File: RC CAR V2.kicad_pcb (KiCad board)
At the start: 2 copper layers, 65 x 65 mm, 62 parts, among them J2 IR1, J3 IR2, J5 US, J6 LW, J7 RW, Q1 S8050, Q2 S8050, SW1 EN, SW2 BOOT, U1 L7805, U2 SRV05-4, U3 AMS1117-3.3, U4 CH340K, U6 L293DD, U7 ESP32-WROOM-32D

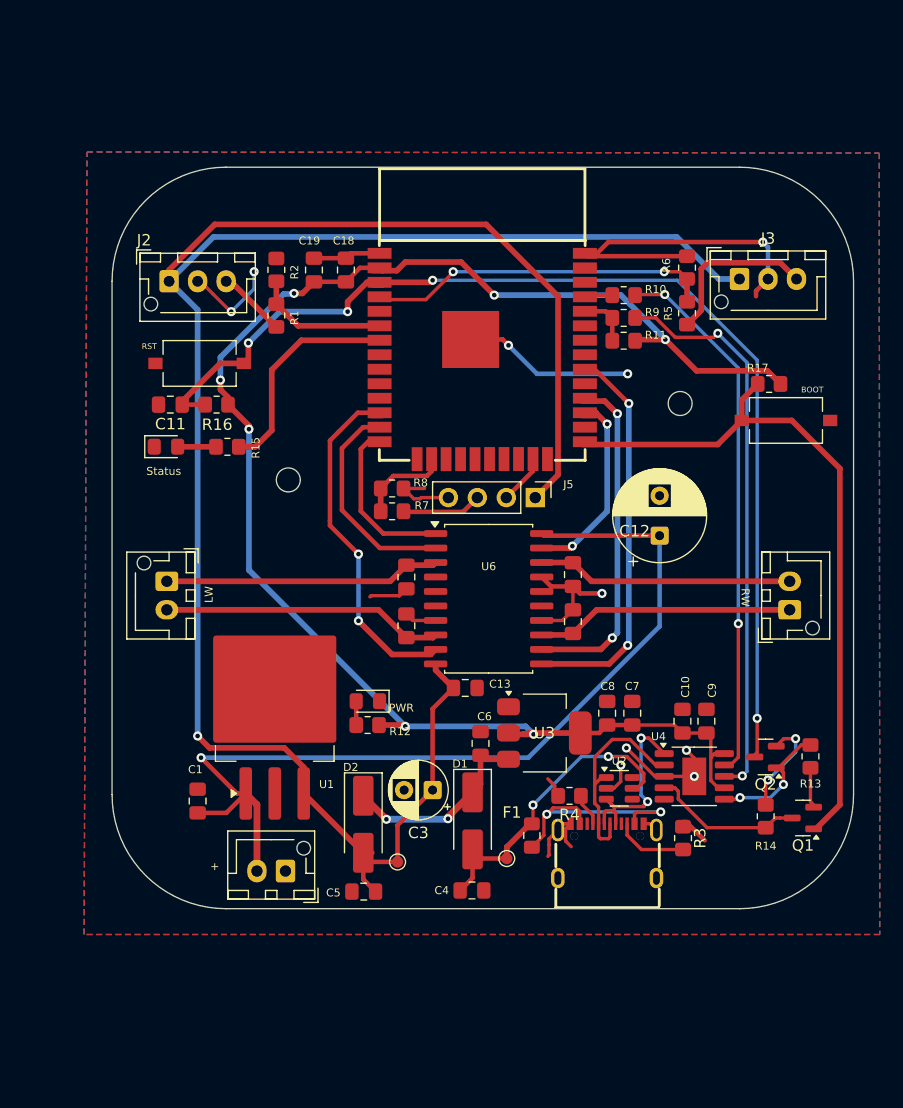
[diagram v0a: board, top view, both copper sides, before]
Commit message: Version of the RC_CAR Circuit Routing Done
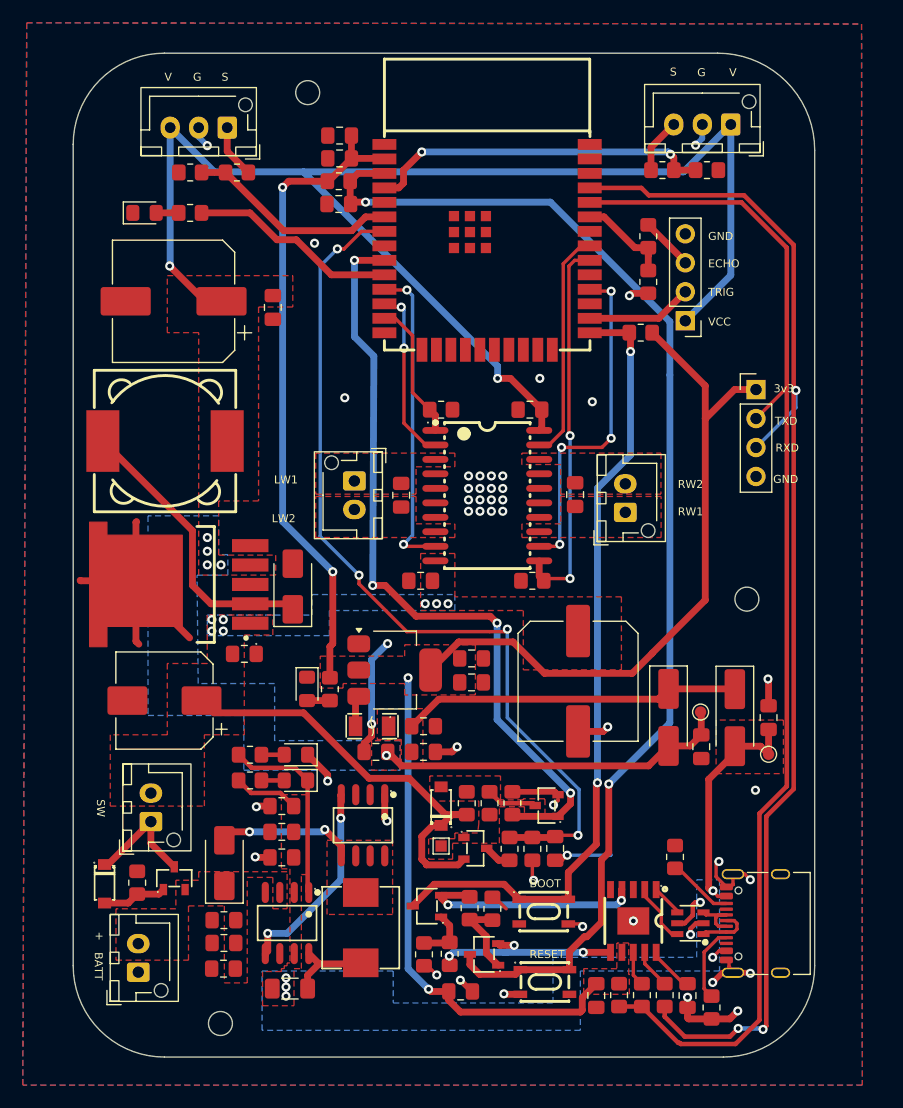
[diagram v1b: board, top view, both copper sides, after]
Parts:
- removed H1: MountingHole, MountingHole:MountingHole_2.1mm
- removed Q2: S8050, Package_TO_SOT_SMD:SOT-23
- removed R3, R4: 5k1, Resistor_SMD:R_0805_2012Metric_Pad1.20x1.40mm_HandSolder
- removed SW1: EN, Button_Switch_SMD:SW_Tactile_SPST_NO_Straight_CK_PTS636Sx25SMTRLFS
- removed SW2: BOOT, Button_Switch_SMD:SW_Tactile_SPST_NO_Straight_CK_PTS636Sx25SMTRLFS
- removed U7: ESP32-WROOM-32D, EasyEDA:WIFIM-SMD_39P-L25.5-W18.0-P1.27-BL
- removed USB1: TYPE-C 16PIN 2MD, EasyEDA:USB-C-SMD_TYPE-C-16PIN-2MD-073
- added C2: 22uF, Capacitor_SMD:C_0805_2012Metric_Pad1.18x1.45mm_HandSolder, F.Cu at (128.8, 120.6)
- added C20: 100nF, Capacitor_SMD:C_0805_2012Metric_Pad1.18x1.45mm_HandSolder, F.Cu at (150.6, 83.6)
- added C21: 22uF, Capacitor_SMD:C_0805_2012Metric_Pad1.18x1.45mm_HandSolder, F.Cu at (133.9, 59.6)
- added C22: 100nF, Capacitor_SMD:C_0805_2012Metric_Pad1.18x1.45mm_HandSolder, F.Cu at (154.5, 91.0)
- added C23: 1uF, Capacitor_SMD:C_0805_2012Metric_Pad1.18x1.45mm_HandSolder, F.Cu at (133.8, 65.6)
- added C24: 100nF, Capacitor_SMD:C_0805_2012Metric_Pad1.18x1.45mm_HandSolder, F.Cu at (139.3, 91.1)
- added C25: 22u, Capacitor_SMD:C_0805_2012Metric_Pad1.18x1.45mm_HandSolder, F.Cu at (171.5, 110.6)
- added C26: 100nF, Capacitor_SMD:C_0805_2012Metric_Pad1.18x1.45mm_HandSolder, F.Cu at (144.5, 134.6)
- added C27: 100nF, Capacitor_SMD:C_0805_2012Metric_Pad1.18x1.45mm_HandSolder, F.Cu at (156.4, 135.0)
- added C28: 22u, Capacitor_SMD:C_0805_2012Metric_Pad1.18x1.45mm_HandSolder, F.Cu at (165.6, 113.1)
- added C32: 100nF, Capacitor_SMD:C_0805_2012Metric_Pad1.18x1.45mm_HandSolder, F.Cu at (164.4, 135.0)
- added D10: SS34, Diode_SMD:D_SMA_Handsoldering, F.Cu at (168.5, 110.6)
- added D11: SS34, Diode_SMD:D_SMA_Handsoldering, F.Cu at (162.7, 110.6)
- added D5: SS34, Diode_SMD:D_SMA, F.Cu at (123.8, 123.3)
- added D6: LED, LED_SMD:LED_0805_2012Metric_Pad1.15x1.40mm_HandSolder, F.Cu at (131.0, 108.1)
- added D7: LED, LED_SMD:LED_0805_2012Metric_Pad1.15x1.40mm_HandSolder, F.Cu at (116.8, 66.3)
- added H2: MountingHole, MountingHole:MountingHole_2.1mm, F.Cu at (169.6, 100.2)
- added H3: MountingHole, MountingHole:MountingHole_2.1mm, F.Cu at (131.1, 55.8)
- added J1: USB_C_Receptacle_USB2.0_16P, Connector_USB:USB_C_Receptacle_Palconn_UTC16-G, F.Cu at (170.3, 128.6)
- added J4: US, Connector_PinHeader_2.54mm:PinHeader_1x04_P2.54mm_Vertical, F.Cu at (164.2, 75.8)
- added L1: CDRH127N-470M, EasyEDA:IND-SMD_L12.3-W12.3, F.Cu at (118.6, 86.3)
- added L2: MHCI06030-4R7M-R8, EasyEDA:IND-SMD_L7.3-W6.6_MHCI06030, F.Cu at (135.8, 129.0)
- added Q3: AO3401A, EasyEDA:SOT-23-3_L2.9-W1.3-P1.90-LS2.4-BR, F.Cu at (145.8, 122.0)
- added Q4: AO3400A, EasyEDA:SOT-23-3_L2.9-W1.3-P1.90-LS2.4-BR, F.Cu at (152.0, 118.3)
- added Q5: S8050H 200-350, EasyEDA:SOT-23-3_L2.9-W1.6-P1.90-LS2.8-BR, F.Cu at (141.6, 127.1)
- added Q6: S8050H 200-350, EasyEDA:SOT-23-3_L2.9-W1.6-P1.90-LS2.8-BR, F.Cu at (146.6, 131.3)
- added Q7: AO3401A, EasyEDA:SOT-23-3_L2.9-W1.3-P1.90-LS2.4-BR, F.Cu at (119.4, 124.7)
- added R18: 1k, Resistor_SMD:R_0805_2012Metric_Pad1.20x1.40mm_HandSolder, F.Cu at (124.9, 62.8)
- added R19: 2k, Resistor_SMD:R_0805_2012Metric_Pad1.20x1.40mm_HandSolder, F.Cu at (120.8, 62.8)
- added R20: 33R, Resistor_SMD:R_0805_2012Metric_Pad1.20x1.40mm_HandSolder, F.Cu at (160.4, 134.9)
- added R21: 33R, Resistor_SMD:R_0805_2012Metric_Pad1.20x1.40mm_HandSolder, F.Cu at (162.4, 134.9)
- added R22: 1k, Resistor_SMD:R_0805_2012Metric_Pad1.20x1.40mm_HandSolder, F.Cu at (161.0, 68.4)
- added R23: 2k, Resistor_SMD:R_0805_2012Metric_Pad1.20x1.40mm_HandSolder, F.Cu at (161.0, 72.4)
- added R24: 100K, Resistor_SMD:R_0805_2012Metric_Pad1.20x1.40mm_HandSolder, F.Cu at (147.3, 127.3)
- added R25: 100K, Resistor_SMD:R_0805_2012Metric_Pad1.20x1.40mm_HandSolder, F.Cu at (141.3, 131.3)
- added R26: 10k, Resistor_SMD:R_0805_2012Metric_Pad1.20x1.40mm_HandSolder, F.Cu at (158.4, 134.9)
- added R27: 10K, Resistor_SMD:R_0805_2012Metric_Pad1.20x1.40mm_HandSolder, F.Cu at (143.5, 131.3)
- added R28: 10K, Resistor_SMD:R_0805_2012Metric_Pad1.20x1.40mm_HandSolder, F.Cu at (145.3, 127.3)
- added R29: 5k1, Resistor_SMD:R_0805_2012Metric_Pad1.20x1.40mm_HandSolder, F.Cu at (163.3, 122.8)
- added R30: 10k, Resistor_SMD:R_0805_2012Metric_Pad1.20x1.40mm_HandSolder, F.Cu at (142.8, 83.6)
- added R31: 10k, Resistor_SMD:R_0805_2012Metric_Pad1.20x1.40mm_HandSolder, F.Cu at (150.8, 98.6)
- added R32: 5k1, Resistor_SMD:R_0805_2012Metric_Pad1.20x1.40mm_HandSolder, F.Cu at (166.5, 136.0)
- added SW3: BOOT, EasyEDA:SW-SMD_4P-L4.2-W3.4-P2.15-LS5.2, F.Cu at (151.8, 127.6)
- added SW4: EN, EasyEDA:SW-SMD_4P-L4.2-W3.4-P2.15-LS5.2, F.Cu at (151.9, 133.8)
- added Switch_Connector1: J3, Connector_JST:JST_XH_B2B-XH-AM_1x02_P2.50mm_Vertical, F.Cu at (117.4, 119.7)
- added TP4: TestPoint, TestPoint:TestPoint_Pad_D1.0mm, F.Cu at (165.5, 110.1)
- added U5: L293DDM/TR, EasyEDA:SOP-20_L12.8-W7.5-P1.27-LS10.4-BL, F.Cu at (146.8, 91.1)
- added ZD1: BZT52C10, EasyEDA:SOD-123_L2.8-W1.8-LS3.7-RD, F.Cu at (142.8, 118.3)
- added ZD2: BZT52C10, EasyEDA:SOD-123_L2.8-W1.8-LS3.7-RD, F.Cu at (113.3, 125.2)
- C1, C10, C16, C9: value 0.1uF -> 22uF
- C11: value 0.1uF -> 22u
- C12: value 470uF -> 10uF; footprint Capacitor_THT:CP_Radial_D8.0mm_P3.50mm -> Capacitor_SMD:C_0805_2012Metric_Pad1.18x1.45mm_HandSolder
- C13, C14, C15, C18: value 0.1uF -> 100nF
- C17: value 0.1uF -> 470uF; footprint Capacitor_SMD:C_0805_2012Metric_Pad1.18x1.45mm_HandSolder -> Capacitor_SMD:C_Elec_10x10.2
- C19: value 22uF -> 100nF
- C3: value CPS -> 100uF; footprint Capacitor_THT:CP_Radial_D5.0mm_P2.50mm -> Capacitor_SMD:CP_Elec_8x10
- C4, C8: value 22u -> 22uF
- C5: value 22u -> 100nF
- C6: value 10u -> 330uF; footprint Capacitor_SMD:C_0805_2012Metric_Pad1.18x1.45mm_HandSolder -> Capacitor_SMD:CP_Elec_10x10.5
- C7: value 0.1u -> 100nF
- D1: value SS34 -> R_LED; footprint Diode_SMD:D_SMA_Handsoldering -> LED_SMD:LED_0805_2012Metric_Pad1.15x1.40mm_HandSolder
- D2: value SS34 -> G_LED; footprint Diode_SMD:D_SMA_Handsoldering -> LED_SMD:LED_0805_2012Metric_Pad1.15x1.40mm_HandSolder
- D3: value LED -> SS34; footprint LED_SMD:LED_0805_2012Metric_Pad1.15x1.40mm_HandSolder -> Diode_SMD:D_SMA
- D4: value LED -> USBLC6-2SC6; footprint LED_SMD:LED_0805_2012Metric_Pad1.15x1.40mm_HandSolder -> EasyEDA:SOT-23-6_L2.9-W1.6-P0.95-LS2.8-BL
- F1: value Polyfuse_Small -> SMD1206P100TF; footprint Fuse:Fuse_0805_2012Metric_Pad1.15x1.40mm_HandSolder -> EasyEDA:F1206
- J5: value US -> LW; footprint Connector_PinHeader_2.54mm:PinHeader_1x04_P2.54mm_Vertical -> Connector_JST:JST_XH_B2B-XH-AM_1x02_P2.50mm_Vertical
- J6: value LW -> RW
- J7: value RW -> Progmmer; footprint Connector_JST:JST_XH_B2B-XH-AM_1x02_P2.50mm_Vertical -> Connector_PinHeader_2.54mm:PinHeader_1x04_P2.54mm_Vertical
- Q1: value S8050 -> AO4468; footprint Package_TO_SOT_SMD:SOT-23 -> EasyEDA:SOP-8_L4.9-W3.9-P1.27-LS6.0-BL
- R1: value 1k -> 4k7
- R10, R9: value 33R -> 10K
- R11: value 10k -> 10K
- R13: value 10K -> 1k
- R14: value 10K -> 10k
- R15: value 1k -> 10k
- R16: value 10k -> 1k
- R17: value 10k -> 2k
- R2: value 2k -> 4k7
- R5: value 1k -> R040; footprint Resistor_SMD:R_0805_2012Metric_Pad1.20x1.40mm_HandSolder -> Resistor_SMD:R_1206_3216Metric_Pad1.30x1.75mm_HandSolder
- R6: value 2k -> 1K
- R7: value 1k -> 430K
- R8: value 2k -> 100K
- TP2: footprint TestPoint:TestPoint_Pad_D1.0mm -> TestPoint:TestPoint_Pad_1.0x1.0mm
- U1: value L7805 -> LM2596SX-5.0/NOPB; footprint Package_TO_SOT_SMD:TO-263-3_TabPin2 -> EasyEDA:TO-263-5_L10.2-W8.9-P1.70-TL
- U2: value SRV05-4 -> CN3303; footprint Package_TO_SOT_SMD:SOT-23-6 -> EasyEDA:SOP-8_L4.9-W3.9-P1.27-LS6.0-BL-1
- U4: value CH340K -> ESP32-WROOM-32E-N8R2; footprint Package_SO:SSOP-10-1EP_3.9x4.9mm_P1mm_EP2.1x3.3mm -> EasyEDA:WIFI-SMD_ESP32-WROOM-32E
- U6: value L293DD -> CH340K; footprint Package_SO:SOIC-20W_7.5x12.8mm_P1.27mm -> EasyEDA:ESOP-10_L4.9-W3.9-P1.00-LS6.2-BL-EP
- moved R6 72.3 mm to (116.2, 125.1)
- moved R13 72.3 mm to (120.8, 66.3), turned to 180 degrees
- moved R5 68.7 mm to (129.5, 134.3), turned to 0 degrees
- moved R14 67.1 mm to (133.8, 63.6), turned to 0 degrees
- moved D4 62.1 mm to (164.6, 128.6), turned to 90 degrees
- moved J2 51.1 mm to (168.2, 58.6), turned to 180 degrees
- moved U4 49.8 mm to (146.8, 69.3), turned to -90 degrees
- moved H4 48.0 mm to (123.5, 137.4)
- moved C7 47.5 mm to (128.0, 74.6)
- moved C6 47.2 mm to (119.3, 74.1), turned to 180 degrees
- moved J3 46.8 mm to (124.0, 58.9), turned to 180 degrees
- moved C9 46.5 mm to (123.8, 130.3), turned to 180 degrees
- moved R10 46.1 mm to (147.0, 118.1), turned to 90 degrees
- moved R9 44.7 mm to (145.0, 118.1), turned to 90 degrees
- moved R16 44.2 mm to (162.2, 62.6), turned to 0 degrees
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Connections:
- BATT1 pad 2: +12V -> /BATT+
- C1 pad 1: +12V -> VBUS
- C10 pad 1: +3.3V -> /BATT+
- C11 pad 1: EN -> +5V
- C12 pad 1: +12V -> V-IN
- C13 pad 1: +5V -> BATT_ADC
- C14 pad 1: RW1 -> V-IN
- C15 pad 1: RW2 -> +3.3V
- C16 pad 1: LW1 -> +3.3V
- C17 pad 1: LW2 -> +12V
- C18 pad 1: +3.3V -> +12V
- C3 pad 1: +5V -> +12V
- C5 pad 1: +5V -> +12V
- C6 pad 1: V-IN -> +5V
- C7 pad 1: +3.3V -> GND
- C7 pad 2: GND -> +5V
- C8 pad 1: +3.3V -> /BATT+
- C9 pad 1: +3.3V -> /BATT+
- D1 pad 1: V-IN -> Net-(D1-K)
- D1 pad 2: VBUS -> Net-(D1-A)
- D2 pad 1: V-IN -> GND
- D2 pad 2: +5V -> Net-(D2-A)
- D3 pad 1: GND -> Net-(D3-K)
- D3 pad 2: Net-(D3-A) -> GND
- D4 pad 1: GND -> D-
- D4 pad 2: Net-(D4-A) -> GND
- F1 pad 1: VBUS -> V-IN
- F1 pad 2: Net-(F1-Pad2) -> Net-(U3-VI)
- J3 pad 1: +5V -> Net-(J3-Pin_1)
- J3 pad 3: Net-(J3-Pin_3) -> +5V
- J5 pad 1: +5V -> LW1
- J5 pad 2: TRIG -> LW2
- J6 pad 1: LW1 -> RW1
- J6 pad 2: LW2 -> RW2
- J7 pad 1: RW1 -> +3.3V
- J7 pad 2: RW2 -> TXD
- Q1 pad 1: IO0 -> GND
- Q1 pad 2: Net-(Q1-B) -> GND
- Q1 pad 3: DTR -> GND
- R1 pad 1: Net-(J2-Pin_3) -> Net-(D1-A)
- R1 pad 2: IR2 -> VBUS
- R10 pad 1: Net-(U4-RXD) -> Net-(Q3-G)
- R10 pad 2: RXD -> Net-(Q3-G)
- R11 pad 1: +3.3V -> BATT_VD_EN
- R11 pad 2: TXD -> GND
- R12 pad 2: Net-(D3-A) -> Net-(D6-A)
- R13 pad 1: RTS -> S_LED
- R13 pad 2: Net-(Q1-B) -> Net-(D7-A)
- R14 pad 1: DTR -> +3.3V
- R14 pad 2: Net-(Q2-B) -> EN
- R15 pad 1: S_LED -> +3.3V
- R15 pad 2: Net-(D4-A) -> IO0
- R16 pad 1: +3.3V -> Net-(J2-Pin_3)
- R16 pad 2: EN -> IR1
- R17 pad 1: +3.3V -> IR1
- R17 pad 2: IO0 -> GND
- R2 pad 1: IR2 -> Net-(D2-A)
- R2 pad 2: GND -> Net-(D1-K)
- R5 pad 1: Net-(J3-Pin_3) -> VBUS
- R5 pad 2: IR1 -> Net-(U2-CSN)
- R6 pad 1: IR1 -> Net-(Q7-G)
- R7 pad 1: Net-(J5-Pin_3) -> Net-(Q3-D)
- R7 pad 2: ECHO -> BATT_ADC
- R8 pad 1: ECHO -> GND
- R8 pad 2: GND -> BATT_ADC
- R9 pad 1: Net-(U4-TXD) -> +12V
- R9 pad 2: TXD -> Net-(Q3-G)
- TP2 pad 1: VBUS -> Net-(Q3-G)
- TP3 pad 1: +5V -> VBUS
- U1 pad 2: GND -> Net-(D3-K)
- U1 pad 3: +5V -> GND
- U2 pad 1: D- -> Net-(D1-K)
- U2 pad 2: GND -> VBUS
- U2 pad 3: D+ -> /BATT+
- U2 pad 4: unconnected-(U2-IO3-Pad4) -> GND
- U2 pad 5: VBUS -> Net-(Q1-G)
- U3 pad 3: V-IN -> Net-(U3-VI)
- U4 pad 1: D+ -> GND
- U4 pad 10: +3.3V -> S_LED
- U4 pad 11: GND -> IN2
- U4 pad 2: D- -> +3.3V
- U4 pad 3: GND -> EN
- U4 pad 4: DTR -> IR1
- U4 pad 6: RTS -> IR2
- U4 pad 7: +3.3V -> BATT_ADC
- U4 pad 8: Net-(U4-TXD) -> unconnected-(U4-IO32-Pad8)
- U4 pad 9: Net-(U4-RXD) -> BATT_VD_EN
- U6 pad 1: ENA -> UD+
- U6 pad 10: +5V -> Net-(U6-V3)
- U6 pad 11: ENB -> GND
- U6 pad 2: IN1 -> UD-
- U6 pad 3: LW1 -> GND
- U6 pad 4: GND -> DTR
- U6 pad 5: GND -> unconnected-(U6-~{CTS}-Pad5)
- U6 pad 6: GND -> RTS
- U6 pad 7: GND -> +3.3V
- U6 pad 8: LW2 -> Net-(U6-TXD)
- U6 pad 9: IN2 -> Net-(U6-RXD)
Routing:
- net RXD: track 2.46 -> 106.8 mm, vias 0 -> 3
- net TXD: track 4.64 -> 106.0 mm
- net BATT_ADC: track 0.00 -> 77.8 mm, vias 0 -> 4
- net BATT_VD_EN: track 0.00 -> 68.2 mm, vias 0 -> 4
- net Net-(U4-TXD): track 49.7 -> 0.00 mm, vias 2 -> 0
- net Net-(U4-RXD): track 47.4 -> 0.00 mm, vias 2 -> 0
- net +5V: track 199.9 -> 152.8 mm, vias 1 -> 7
- net +12V: track 80.7 -> 38.3 mm, vias 1 -> 7
- net Net-(D3-K): track 0.00 -> 25.6 mm
- net LW2: track 24.7 -> 0.00 mm
- net LW1: track 24.2 -> 0.00 mm
- net +3.3V: track 139.4 -> 162.4 mm, vias 7 -> 4
- net RW1: track 22.6 -> 0.00 mm
- net RW2: track 22.4 -> 0.00 mm
- net Net-(F1-Pad2): track 21.1 -> 0.00 mm, vias 2 -> 0
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- added copper zone on B.Cu, net +12V
- added copper zone on F.Cu, net +12V
- added copper zone on F.Cu, net +3.3V
- added copper zone on B.Cu, net +5V
- added copper zone on F.Cu, net +5V
- added copper zone on F.Cu, net /BATT+
- added copper zone on F.Cu, net /Drain
- added copper zone on F.Cu, net LW1
- added copper zone on F.Cu, net LW2
- added copper zone on F.Cu, net Net-(Q3-G)
- added copper zone on F.Cu, net RW1
- added copper zone on F.Cu, net RW2
- added copper zone on F.Cu, net V-IN
- added copper zone on B.Cu, net VBUS
- added copper zone on F.Cu, net VBUS
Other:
- board size 65 x 65 mm -> 65 x 88 mm
- board text added: "3v3"
- board text added: "BATT"
- board text added: "ECHO"
- board text added: "G"
- board text added: "GND"
- board text added: "LW1"
- board text added: "LW2"
- board text added: "RESET"
- board text added: "RW1"
- board text added: "RW2"
- board text added: "RXD"
- board text added: "S"
- board text added: "SW"
- board text added: "TRIG"
- board text added: "TXD"
- board text added: "V"
- board text added: "VCC"
- board text removed: "LW"
- board text removed: "PWR"
- board text removed: "RST"
- board text removed: "RW"
- board text removed: "Status"
